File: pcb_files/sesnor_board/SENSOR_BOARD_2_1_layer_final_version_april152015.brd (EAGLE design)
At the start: 131.8 x 60.5 mm, 7 parts

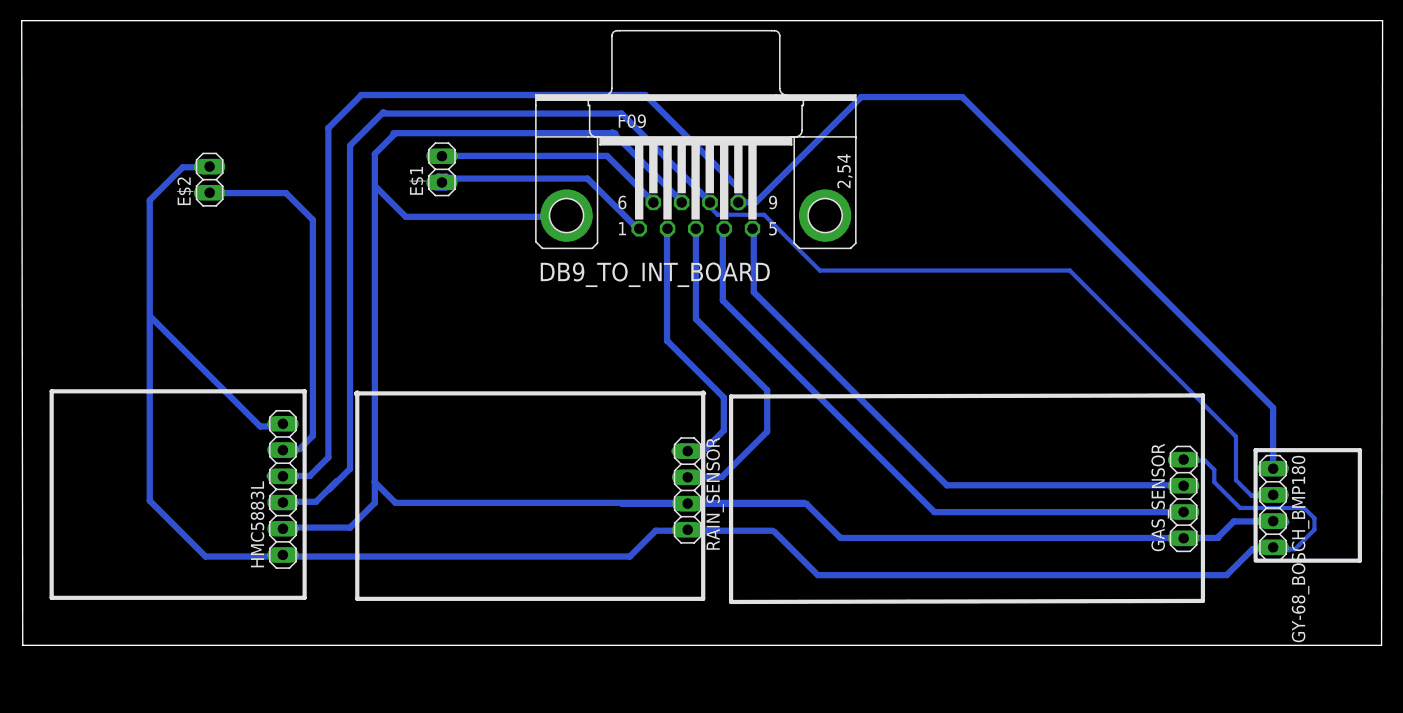
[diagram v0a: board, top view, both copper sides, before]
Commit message: Sensor_board and Main Board Update
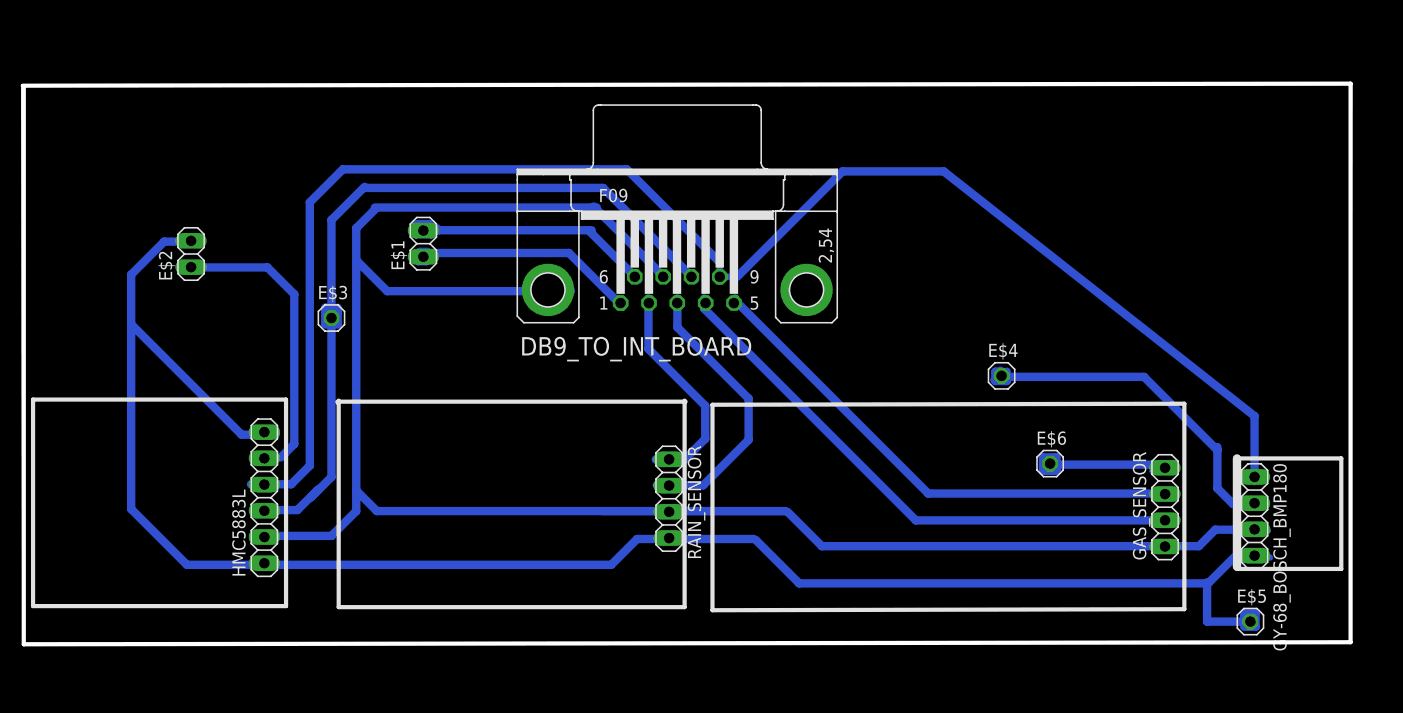
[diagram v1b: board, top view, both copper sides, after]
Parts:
- added E$3, E$4, E$5, E$6: (no value), pinhead:1X01
- moved E$1 7.42 mm to (38.8, 38.9)
- moved E$2 7.42 mm to (16.3, 37.9)
- moved DB9_TO_INT_BOARD 7.42 mm to (63.4, 34.4)
- moved GAS_SENSOR 1.97 mm to (110.6, 13.4)
- moved RAIN_SENSOR 1.97 mm to (62.6, 14.2)
- moved HMC5883L 1.97 mm to (23.4, 14.3)
- moved GY-68_BOSCH_BMP180 1.97 mm to (119.3, 12.5)
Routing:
- net S$20: track 70.3 -> 33.9 mm
- net S$21: track 76.0 -> 52.6 mm
- net S$28: track 0.00 -> 15.3 mm
- net S$32: track 0.00 -> 15.1 mm
- net S$27: track 0.00 -> 12.3 mm
- net S$17: track 89.7 -> 83.3 mm
- net S$7: track 61.5 -> 55.1 mm
- net S$6: track 56.9 -> 50.5 mm
- net S$19: track 27.9 -> 21.5 mm
- net S$5: track 37.5 -> 31.1 mm
- net S$16: track 85.0 -> 78.6 mm
- net S$10: track 38.8 -> 32.4 mm
- net S$18: track 33.7 -> 27.3 mm
- net S$3: track 100.4 -> 94.0 mm
- net S$26: track 0.00 -> 5.80 mm
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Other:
- board size 131.8 x 60.5 mm -> 128.8 x 54.3 mm
